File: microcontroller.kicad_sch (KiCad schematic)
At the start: 0 parts

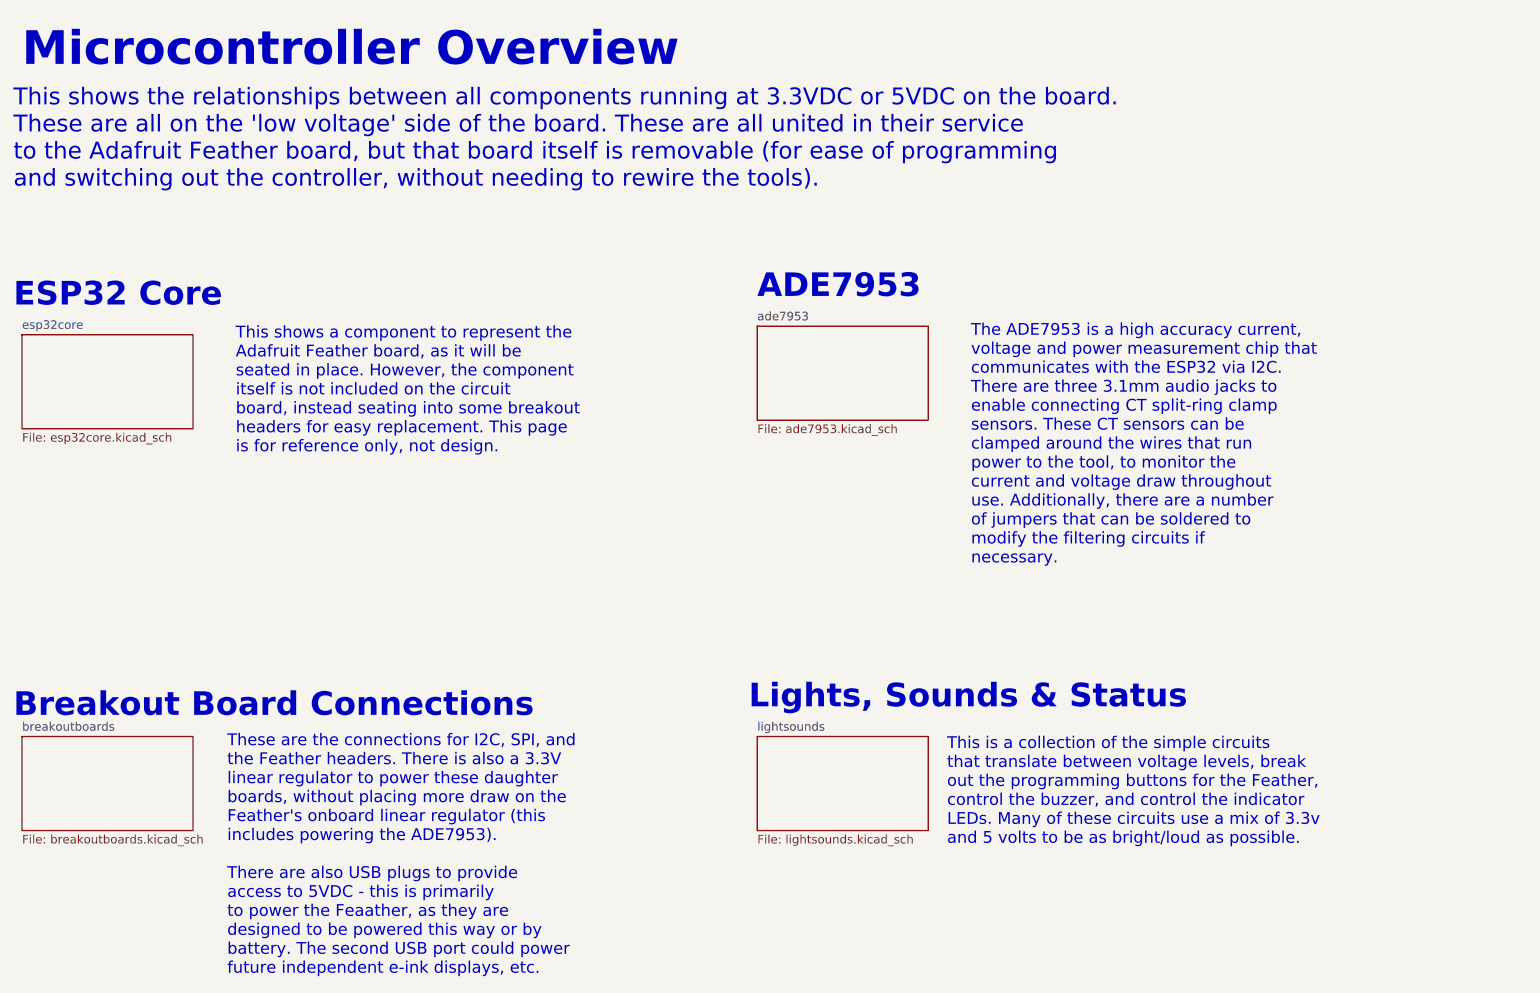
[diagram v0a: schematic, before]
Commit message: 1.4.1 schematic update
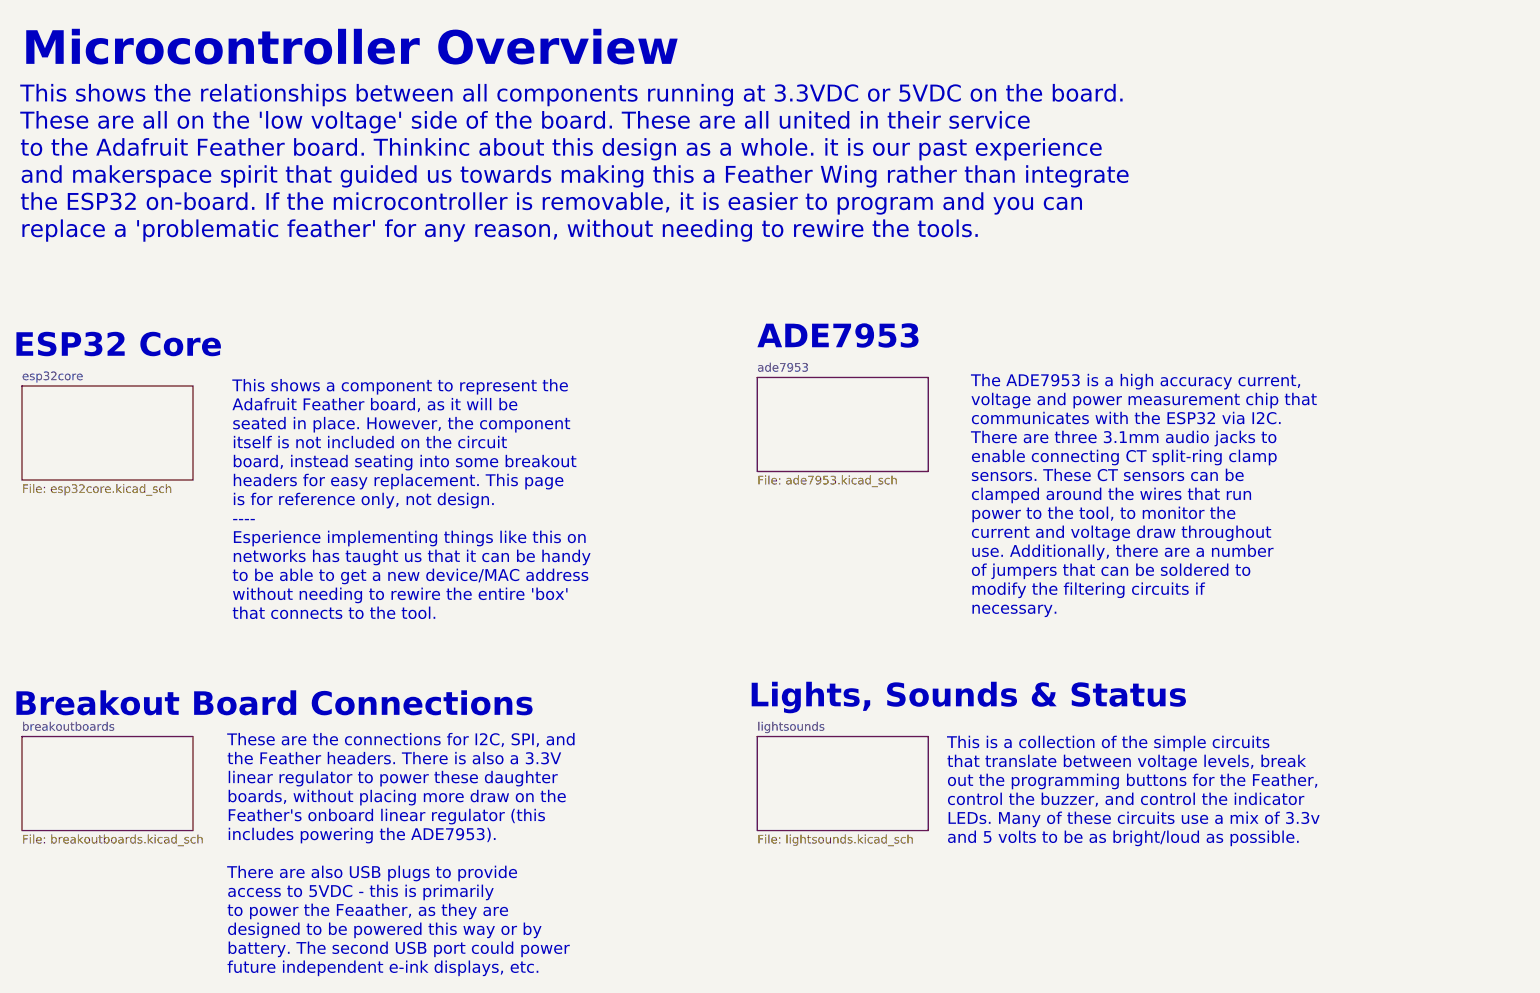
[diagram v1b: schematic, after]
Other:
- note added: "This shows a component to represent the Adafruit Feather board, as it will be seated in place. However, the component itself is not included on the circuit board, instead seating into some breakout headers for easy replacement. This page is for reference only, not design. ---- Esperience implementing things like this on networks has taught us that it can be handy to be able to get a new device/MA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"
- note added: "This shows the relationships between all components running at 3.3VDC or 5VDC on the board. These are all on the 'low voltage' side of the board. These are all united in their service to the Adafruit Feather board. Thinkinc about this design as a whole. it is our past experience and makerspace spirit that guided us towards making this a Feather Wing rather than integrate the ESP32 on-board. If th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"
- note removed: "This shows a component to represent the Adafruit Feather board, as it will be seated in place. However, the component itself is not included on the circuit board, instead seating into some breakout headers for easy replacement. This page is for reference only, not design."
- note removed: "This shows the relationships between all components running at 3.3VDC or 5VDC on the board. These are all on the 'low voltage' side of the board. These are all united in their service to the Adafruit Feather board, but that board itself is removable (for ease of programming and switching out the controller, without needing to rewire the tools)."
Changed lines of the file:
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@@
 		(company "Corey Rice & MakeHaven")
 	)
-	(text "This shows the relationships between all components running at 3.3VDC or 5VDC on the board. \nThese are all on the 'low voltage' side of the board. These are all united in their service \nto the Adafruit Feather board, but that board itself is removable (for ease of programming \nand switching out the controller, without needing to rewire the tools). "
+	(text "This shows the relationships between all components running at 3.3VDC or 5VDC on the board. \nThese are all on the 'low voltage' side of the board. These are all united in their service \nto the Adafruit Feather board. Thinkinc about this design as a whole. it is our past experience\nand makerspace spirit that guided us towards making this a Feather Wing rather than integrate\nthe ESP32 on-board. If the microcontroller is removable, it is easier to program and you can \nreplace a 'problematic feather' for any reason, without needing to rewire the tools. "
 		(exclude_from_sim no)
-		(at 33.02 49.53 0)
+		(at 34.036 57.15 0)
 		(effects
 			(font
@@
 		)
 	)
-	(text "This shows a component to represent the \nAdafruit Feather board, as it will be \nseated in place. However, the component \nitself is not included on the circuit \nboard, instead seating into some breakout \nheaders for easy replacement. This page \nis for reference only, not design."
+	(text "This shows a component to represent the \nAdafruit Feather board, as it will be \nseated in place. However, the component \nitself is not included on the circuit \nboard, instead seating into some breakout \nheaders for easy replacement. This page \nis for reference only, not design.\n----\nEsperience implementing things like this on \nnetworks has taught us that it can be handy\nto be able to get a new device/MAC address \nwithout needing to rewire the entire 'box'\nthat connects to the tool."
 		(exclude_from_sim no)
-		(at 66.04 88.9 0)
+		(at 65.532 113.792 0)
 		(effects
 			(font
@@
 	(text "The ADE7953 is a high accuracy current, \nvoltage and power measurement chip that \ncommunicates with the ESP32 via I2C. \nThere are three 3.1mm audio jacks to \nenable connecting CT split-ring clamp \nsensors. These CT sensors can be \nclamped around the wires that run \npower to the tool, to monitor the \ncurrent and voltage draw throughout \nuse. Additionally, there are a number \nof jumpers that can be soldered to \nmodify the filtering circuits if \nnecessary. "
 		(exclude_from_sim no)
-		(at 175.26 105.41 0)
+		(at 175.26 113.03 0)
 		(effects
 			(font
@@
 	(text "ESP32 Core"
 		(exclude_from_sim no)
-		(at 33.02 67.31 0)
+		(at 33.02 74.93 0)
 		(effects
 			(font
@@
 	(text "ADE7953"
 		(exclude_from_sim no)
-		(at 143.51 66.04 0)
+		(at 143.51 73.66 0)
 		(effects
 			(font
@@
 	)
 	(sheet
-		(at 143.51 69.85)
+		(at 143.51 77.47)
 		(size 25.4 13.97)
 		(fields_autoplaced yes)
@@
 		)
 		(property "Sheetname" "ade7953"
-			(at 143.51 69.1384 0)
+			(at 143.51 76.7584 0)
 			(effects
 				(font
@@
 		)
 		(property "Sheetfile" "ade7953.kicad_sch"
-			(at 143.51 84.4046 0)
+			(at 143.51 92.0246 0)
 			(effects
 				(font
@@
 	)
 	(sheet
-		(at 34.29 71.12)
+		(at 34.29 78.74)
 		(size 25.4 13.97)
 		(fields_autoplaced yes)
@@
 		)
 		(property "Sheetname" "esp32core"
-			(at 34.29 70.4084 0)
+			(at 34.29 78.0284 0)
 			(effects
 				(font
@@
 		)
 		(property "Sheetfile" "esp32core.kicad_sch"
-			(at 34.29 85.6746 0)
+			(at 34.29 93.2946 0)
 			(effects
 				(font
